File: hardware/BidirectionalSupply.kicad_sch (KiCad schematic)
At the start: 0 parts

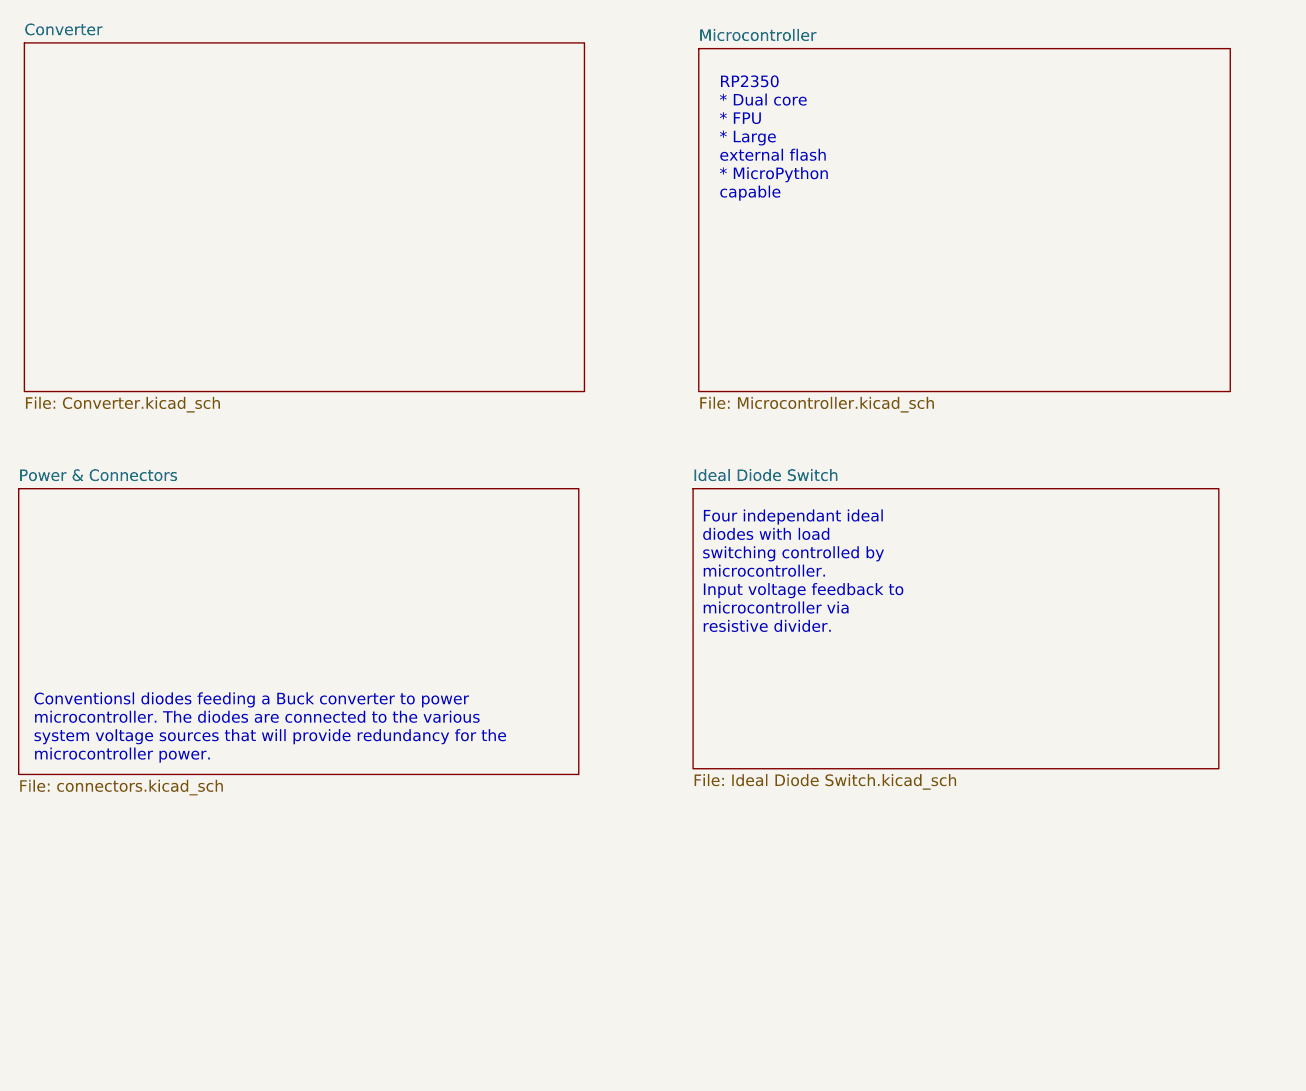
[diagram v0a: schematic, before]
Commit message: Ready for trial submit to JLCPCB
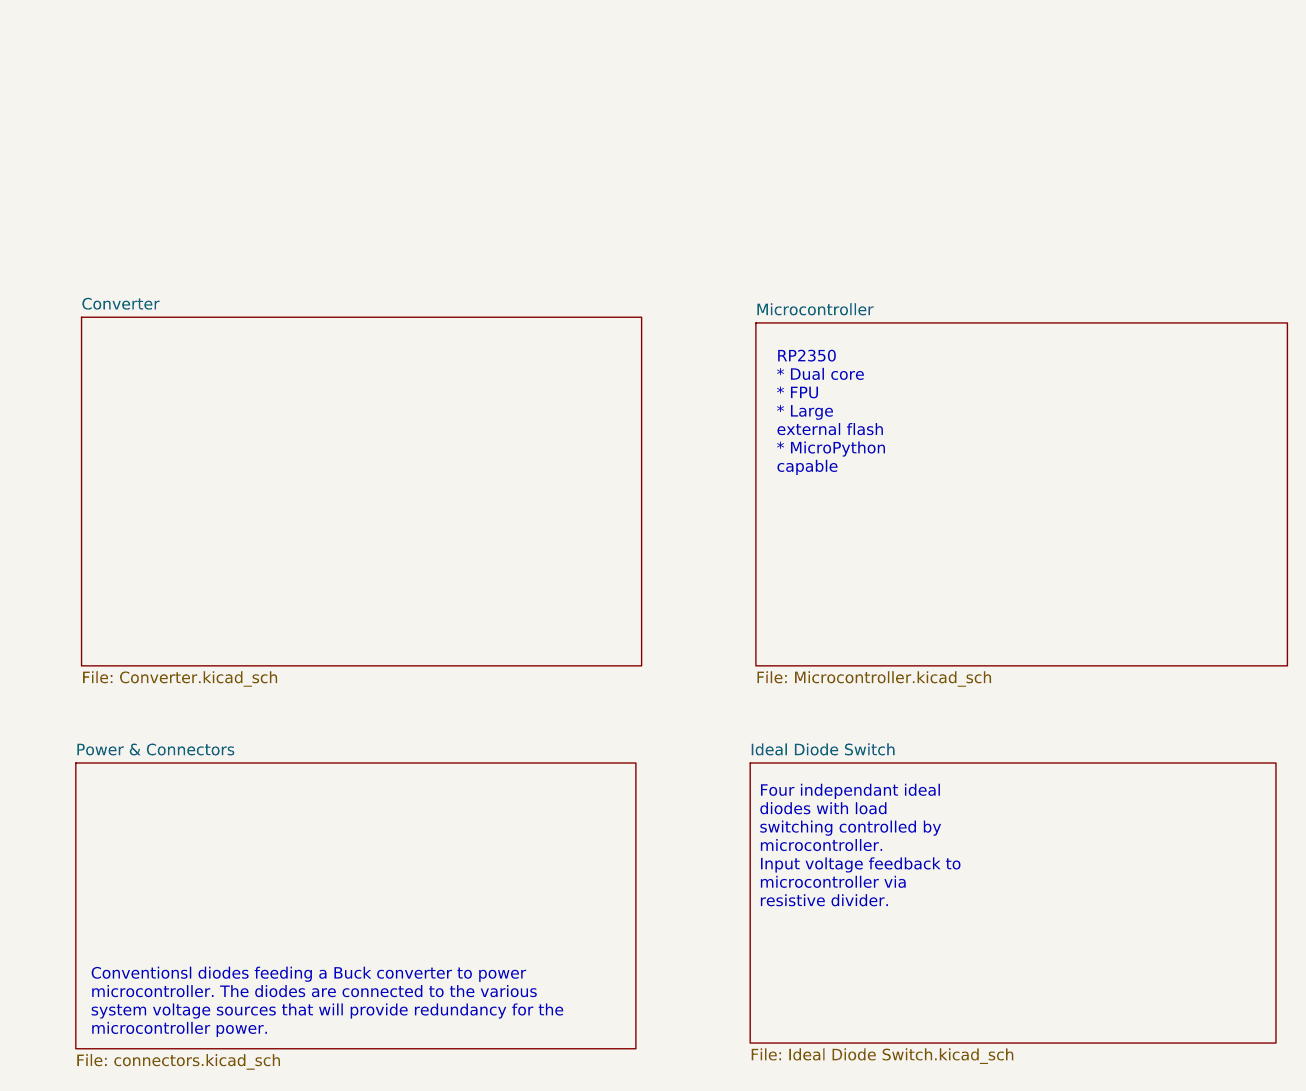
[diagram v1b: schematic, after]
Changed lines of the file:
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@@
 	)
 	(image
-		(at 180.975 40.64)
+		(at 187.325 71.12)
 		(scale 0.786294)
 		(data "/9j/4Q/+RXhpZgAATU0AKgAAAAgABgESAAMAAAABAAEAAAEaAAUAAAABAAAAVgEbAAUAAAABAAAA"
@@
 	)
 	(image
-		(at 100.33 40.64)
+		(at 106.68 71.12)
 		(scale 0.629422)
 		(data "iVBORw0KGgoAAAANSUhEUgAAA+YAAAKoCAYAAAD6ReWPAAABJ2lDQ1BrQ0dDb2xvclNwYWNlQWRv"
@@
 	)
 	(image
-		(at 98.425 81.915)
+		(at 104.775 112.395)
 		(scale 0.287766)
 		(data "iVBORw0KGgoAAAANSUhEUgAAB9IAAANCCAYAAAA6LIcfAAABJ2lDQ1BrQ0dDb2xvclNwYWNlQWRv"
@@
 	)
 	(image
-		(at 184.785 84.455)
+		(at 191.135 114.935)
 		(scale 2.12927)
 		(data "/9j/4QDKRXhpZgAATU0AKgAAAAgABgESAAMAAAABAAEAAAEaAAUAAAABAAAAVgEbAAUAAAABAAAA"
@@
 	(text_box "RP2350\n* Dual core\n* FPU\n* Large external flash\n* MicroPython capable"
 		(exclude_from_sim no)
-		(at 144.145 24.13 0)
+		(at 150.495 54.61 0)
 		(size 17.78 15.24)
 		(stroke
@@
 	(text_box "Four independant ideal diodes with load switching controlled by microcontroller.\nInput voltage feedback to microcontroller via resistive divider."
 		(exclude_from_sim no)
-		(at 142.24 72.39 0)
+		(at 148.59 102.87 0)
 		(size 27.305 13.97)
 		(stroke
@@
 	(text_box "Conventionsl diodes feeding a Buck converter to power microcontroller. The diodes are connected to the various system voltage sources that will provide redundancy for the microcontroller power."
 		(exclude_from_sim no)
-		(at 67.945 92.71 0)
+		(at 74.295 123.19 0)
 		(size 61.595 9.525)
 		(stroke
@@
 	)
 	(sheet
-		(at 142.875 22.225)
+		(at 149.225 52.705)
 		(size 59.055 38.1)
 		(fields_autoplaced yes)
@@
 		)
 		(property "Sheetname" "Microcontroller"
-			(at 142.875 21.5134 0)
+			(at 149.225 51.9934 0)
 			(effects
 				(font
@@
 		)
 		(property "Sheetfile" "Microcontroller.kicad_sch"
-			(at 142.875 60.9096 0)
+			(at 149.225 91.3896 0)
 			(effects
 				(font
@@
 	)
 	(sheet
-		(at 142.24 71.12)
+		(at 148.59 101.6)
 		(size 58.42 31.115)
 		(fields_autoplaced yes)
@@
 		)
 		(property "Sheetname" "Ideal Diode Switch"
-			(at 142.24 70.4084 0)
+			(at 148.59 100.8884 0)
 			(effects
 				(font
@@
 		)
 		(property "Sheetfile" "Ideal Diode Switch.kicad_sch"
-			(at 142.24 102.8196 0)
+			(at 148.59 133.2996 0)
 			(effects
 				(font
@@
 	)
 	(sheet
-		(at 67.31 71.12)
+		(at 73.66 101.6)
 		(size 62.23 31.75)
 		(fields_autoplaced yes)
@@
 		)
 		(property "Sheetname" "Power & Connectors"
-			(at 67.31 70.4084 0)
+			(at 73.66 100.8884 0)
 			(effects
 				(font
@@
 		)
 		(property "Sheetfile" "connectors.kicad_sch"
-			(at 67.31 103.4546 0)
+			(at 73.66 133.9346 0)
 			(effects
 				(font
@@
 	)
 	(sheet
-		(at 67.945 21.59)
+		(at 74.295 52.07)
 		(size 62.23 38.735)
 		(fields_autoplaced yes)
@@
 		)
 		(property "Sheetname" "Converter"
-			(at 67.945 20.8784 0)
+			(at 74.295 51.3584 0)
 			(effects
 				(font
@@
 		)
 		(property "Sheetfile" "Converter.kicad_sch"
-			(at 67.945 60.9096 0)
+			(at 74.295 91.3896 0)
 			(effects
 				(font
